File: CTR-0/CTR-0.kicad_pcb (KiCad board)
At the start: 2 copper layers, 21 x 51 mm, 36 parts, among them J1 USB_C_Receptacle_USB2.0_14P, J2 Conn_01x20, J3 Conn_01x20, J4 Conn_01x03, SW1 SW_Push, SW2 SW_Push, U1 RP2040, U2 NCP1117-3.3_SOT223, U3 W25Q128JVS, Y1 12MHz

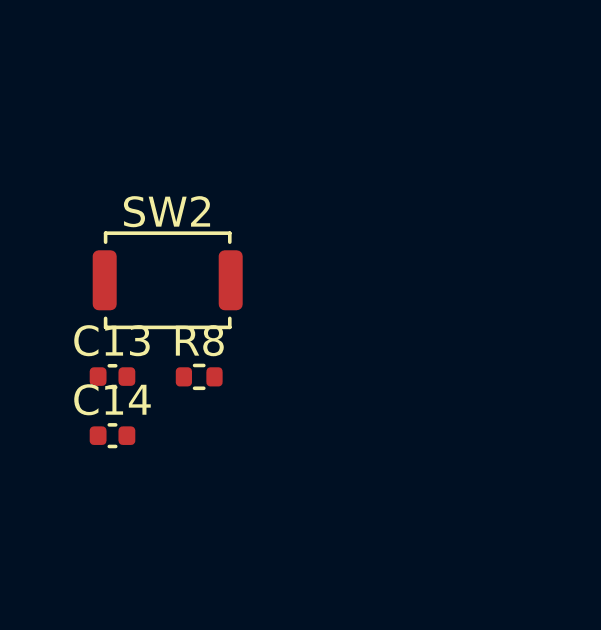
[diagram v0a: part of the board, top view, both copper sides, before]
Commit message: Add files via upload
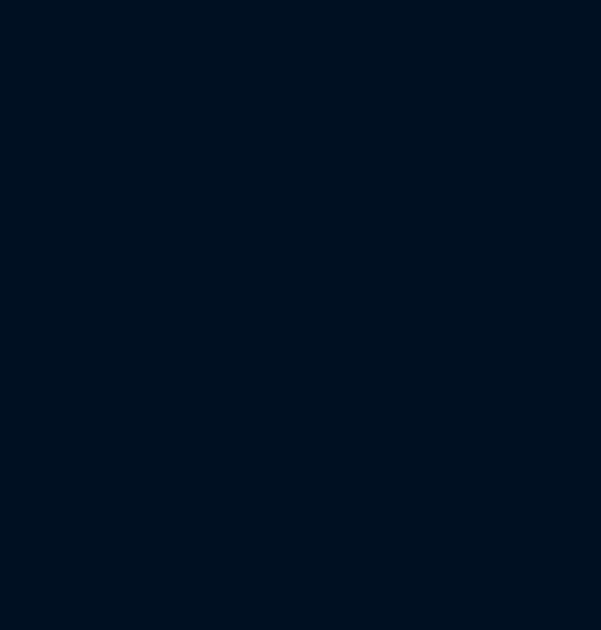
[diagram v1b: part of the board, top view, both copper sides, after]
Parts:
- removed C13, C14: 0.1u, Capacitor_SMD:C_0402_1005Metric
- removed R8: 10k, Resistor_SMD:R_0402_1005Metric
- removed SW2: SW_Push, Button_Switch_SMD:SW_Push_SPST_NO_Alps_SKRK
- C3, C4: value 15p -> 33p
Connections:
- C1 pad 1: +5V -> VBUS
- J1 pad A4: +5V -> VBUS
- J1 pad A9: +5V -> VBUS
- J1 pad B4: +5V -> VBUS
- J1 pad B9: +5V -> VBUS
- J3 pad 1: +3V3 -> VBUS
- J3 pad 10: /GPIO24 -> /GPIO23
- J3 pad 11: /GPIO23 -> /RUN
- J3 pad 9: /GPIO25 -> /GPIO24
- U1 pad 26: Net-(U1-RUN) -> /RUN
- U1 pad 37: /GPIO25 -> unconnected-(U1-GPIO25-Pad37)
- U2 pad 3: +5V -> VBUS

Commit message: fixed push
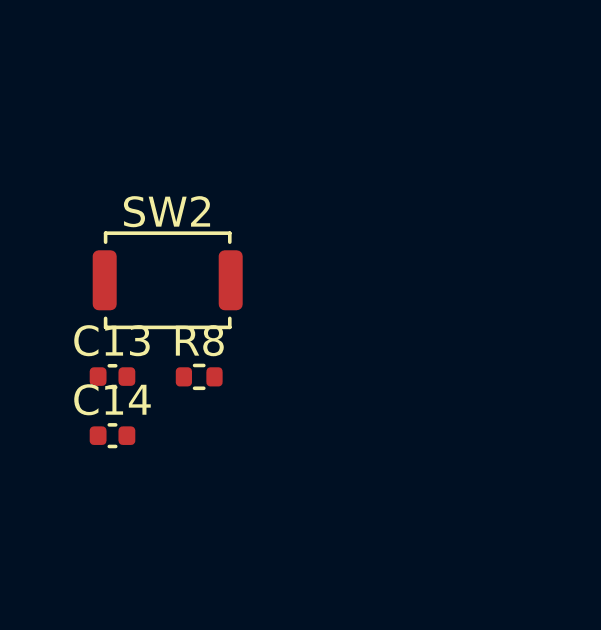
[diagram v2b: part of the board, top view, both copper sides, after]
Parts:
- added C13: 0.1u, Capacitor_SMD:C_0402_1005Metric, F.Cu at (161.4, 89.2)
- added C14: 0.1u, Capacitor_SMD:C_0402_1005Metric, F.Cu at (161.4, 91.1)
- added R8: 10k, Resistor_SMD:R_0402_1005Metric, F.Cu at (164.3, 89.2)
- added SW2: SW_Push, Button_Switch_SMD:SW_Push_SPST_NO_Alps_SKRK, F.Cu at (163.2, 86.0)
- C3, C4: value 33p -> 15p
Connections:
- C1 pad 1: VBUS -> +5V
- J1 pad A4: VBUS -> +5V
- J1 pad A9: VBUS -> +5V
- J1 pad B4: VBUS -> +5V
- J1 pad B9: VBUS -> +5V
- J3 pad 1: VBUS -> +3V3
- J3 pad 10: /GPIO23 -> /GPIO24
- J3 pad 11: /RUN -> /GPIO23
- J3 pad 9: /GPIO24 -> /GPIO25
- U1 pad 26: /RUN -> Net-(U1-RUN)
- U1 pad 37: unconnected-(U1-GPIO25-Pad37) -> /GPIO25
- U2 pad 3: VBUS -> +5V
